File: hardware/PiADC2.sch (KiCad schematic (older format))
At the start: 1 part

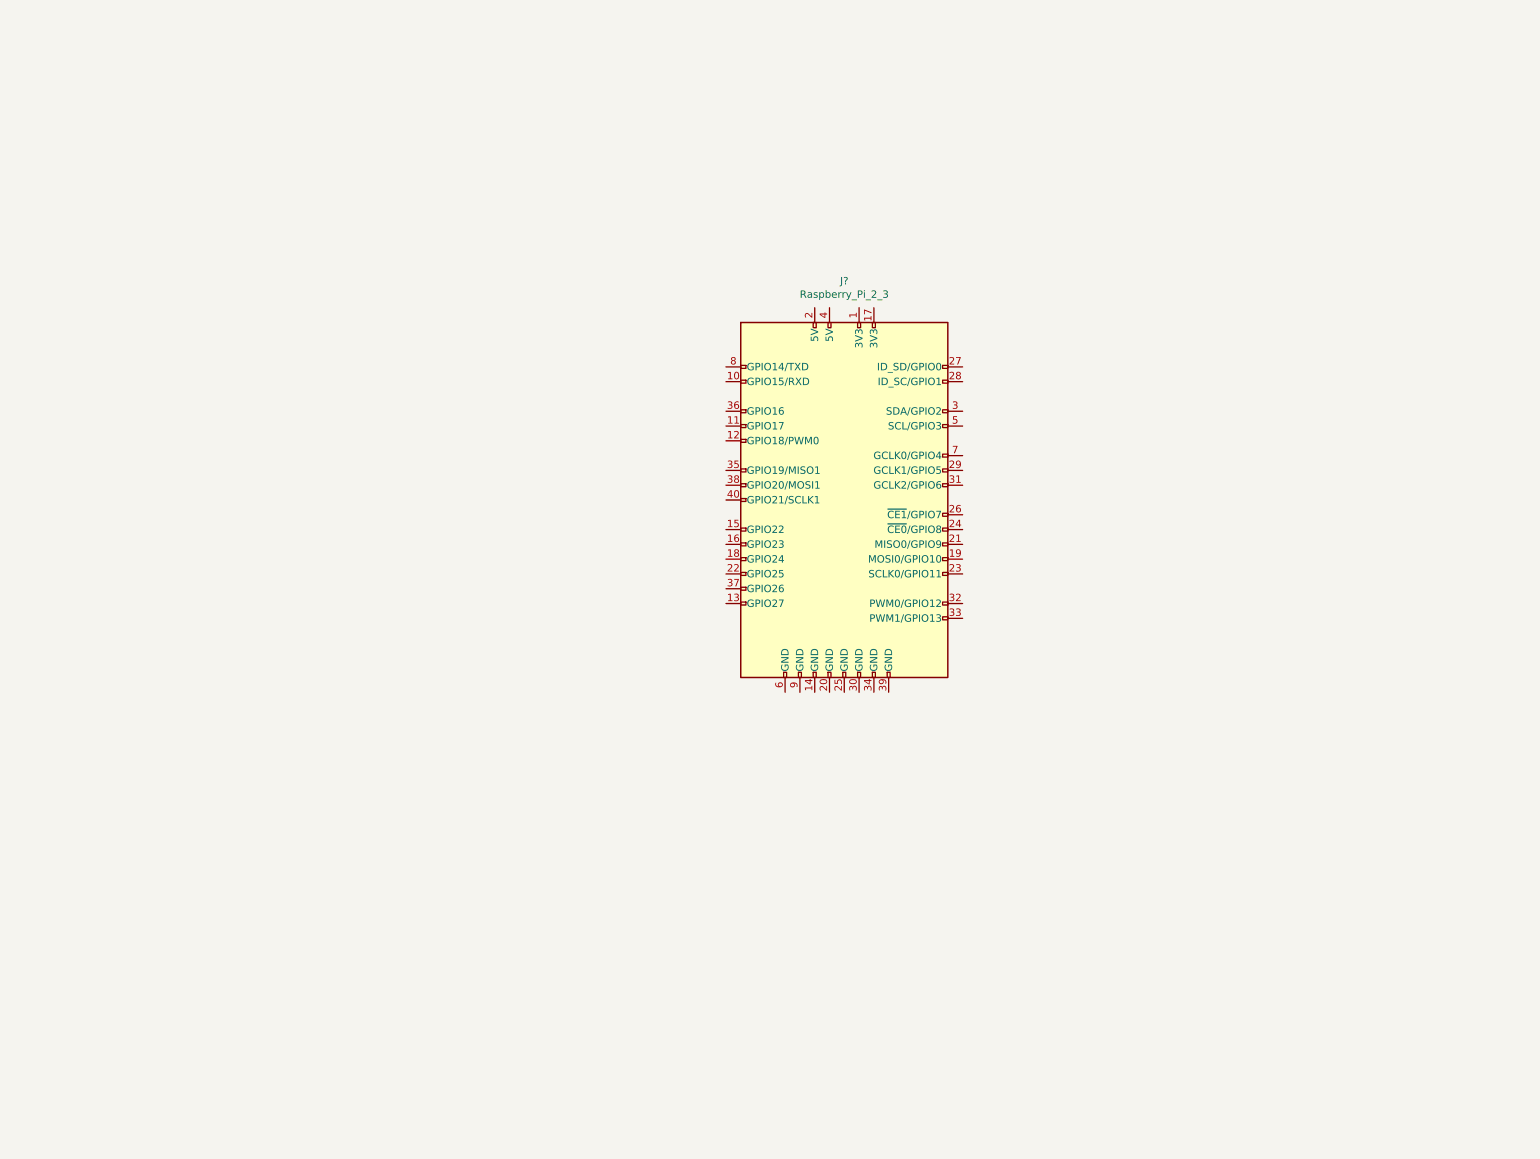
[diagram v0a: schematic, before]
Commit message: Completed version 1
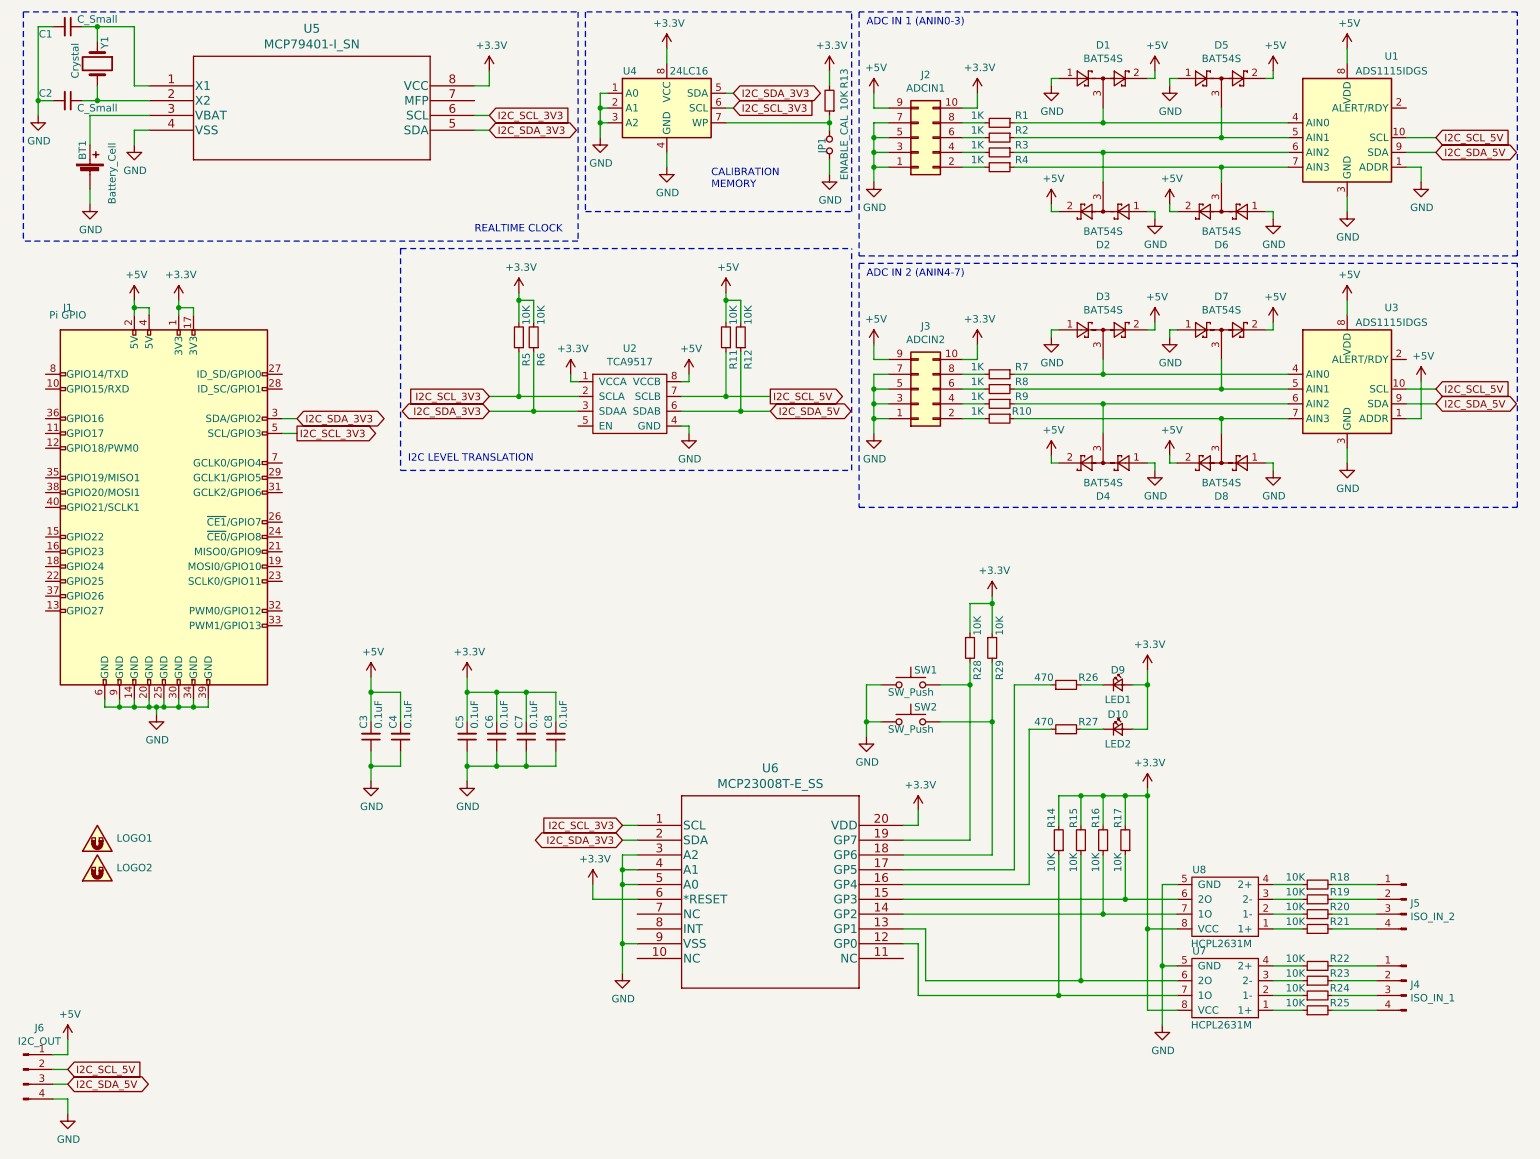
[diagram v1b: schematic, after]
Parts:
- added BT1: Battery_Cell, BH401:BH401, symbol Device:Battery_Cell
- added C1, C2: C_Small, Capacitor_SMD:C_0603_1608Metric, symbol Device:C_Small
- added C3, C4, C5, C6, C7, C8: 0.1uF, Capacitor_SMD:C_0603_1608Metric, symbol Device:C_Small
- added D1, D2, D3, D4, D5, D6, D7, D8: BAT54S, Package_TO_SOT_SMD:SOT-23, symbol Diode:BAT54S
- added D10: LED2, LED_SMD:LED_0603_1608Metric, symbol Device:LED_Small
- added D9: LED1, LED_SMD:LED_0603_1608Metric, symbol Device:LED_Small
- added J2: ADCIN1, Connector_JST:JST_PUD_B10B-PUDSS_2x05_P2.00mm_Vertical, symbol Connector_Generic:Conn_02x05_Odd_Even
- added J3: ADCIN2, Connector_JST:JST_PUD_B10B-PUDSS_2x05_P2.00mm_Vertical, symbol Connector_Generic:Conn_02x05_Odd_Even
- added J4: ISO_IN_1, JST-XA:B04B-XASK-1(LF)(SN), symbol Connector:Conn_01x04_Male
- added J5: ISO_IN_2, JST-XA:B04B-XASK-1(LF)(SN), symbol Connector:Conn_01x04_Male
- added J6: I2C_OUT, Connector_PinHeader_2.54mm:PinHeader_1x04_P2.54mm_Vertical, symbol Connector:Conn_01x04_Male
- added JP1: ENABLE_CAL, Connector_PinHeader_1.27mm:PinHeader_1x02_P1.27mm_Vertical, symbol Device:Jumper_NO_Small
- added LOGO1: SYM_Magnet_Small, CapConiX_Logos:CapConiX_Logo_10_7, symbol Graphic:SYM_Magnet_Small
- added LOGO2: SYM_Magnet_Small, Symbol:OSHW-Logo_5.7x6mm_SilkScreen, symbol Graphic:SYM_Magnet_Small
- added R1, R10, R2, R3, R4, R7, R8, R9: 1K, Resistor_SMD:R_0603_1608Metric, symbol Device:R_Small
- added R11, R12, R13, R14, R15, R16, R17, R18, R19, R20, R21, R22, R23, R24, R25, R28, R29, R5, R6: 10K, Resistor_SMD:R_0603_1608Metric, symbol Device:R_Small
- added R26, R27: 470, Resistor_SMD:R_0603_1608Metric, symbol Device:R_Small
- added SW1, SW2: SW_Push, Button_Switch_SMD:SW_SPST_TL3305A, symbol Switch:SW_Push
- added U1, U3: ADS1115IDGS, Package_SO:TSSOP-10_3x3mm_P0.5mm, symbol Analog_ADC:ADS1115IDGS
- added U2: TCA9517, Package_SO:MSOP-8_3x3mm_P0.65mm, symbol tca9517:TCA9517
- added U4: 24LC16, Package_SO:SO-8_3.9x4.9mm_P1.27mm, symbol Memory_EEPROM:24LC16
- added U5: MCP79401-I_SN, Package_SO:SO-8_3.9x4.9mm_P1.27mm, symbol MCP79401:MCP79401-I_SN
- added U6: MCP23008T-E_SS, Package_SO:SSOP-20_5.3x7.2mm_P0.65mm, symbol MCP23008:MCP23008T-E_SS
- added U7, U8: HCPL2631M, Package_DIP:DIP-8_W7.62mm_LongPads, symbol HCPL2631M:HCPL2631M
- added Y1: Crystal, Crystal:Crystal_DS26_D2.0mm_L6.0mm_Horizontal_1EP_style2, symbol Device:Crystal
- J1: renamed from J?; value Raspberry_Pi_2_3 -> Pi GPIO; footprint (none) -> raspberry_pi:pi_b_hat
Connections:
- net +3V3: now reaches J1.1 (3V3)
- net +3V3: now also J1.17 (3V3), C5.2, C6.2, C7.2, C8.2, D10.2 (A), D9.2 (A), J2.10 (Pin_10), J3.10 (Pin_10), R13.2, R14.2, R15.2, R16.2, R17.2, R28.1, R29.1, R5.2, R6.2, U2.1 (VCCA), U4.8 (VCC), U5.8 (VCC), U6.20 (VDD), U6.6 (*RESET), U7.8 (VCC), U8.8 (VCC)
- net GND: now reaches J1.14 (GND)
- net GND: now also J1.20 (GND), J1.25 (GND), J1.30 (GND), J1.34 (GND), J1.39 (GND), J1.6 (GND), J1.9 (GND), BT1.2 (-), C1.2, C2.2, C3.1, C4.1, C5.1, C6.1, C7.1, C8.1, D1.1, D2.1, D3.1, D4.1, D5.1, D6.1, D7.1, D8.1, J2.1 (Pin_1), J2.3 (Pin_3), J2.5 (Pin_5), J2.7 (Pin_7), J3.1 (Pin_1), J3.3 (Pin_3), J3.5 (Pin_5), J3.7 (Pin_7), J6.4 (Pin_4), JP1.2, SW1.1, SW2.1, U1.1 (ADDR), U1.3 (GND), U2.4 (GND), U3.3 (GND), U4.1 (A0), U4.2 (A1), U4.3 (A2), U4.4 (GND), U5.4 (VSS), U6.3 (A2), U6.4 (A1), U6.5 (A0), U6.9 (VSS), U7.5 (GND), U8.5 (GND)
- net +5V: now reaches J1.2 (5V)
- net +5V: now also J1.4 (5V), C3.2, C4.2, D1.2, D2.2, D3.2, D4.2, D5.2, D6.2, D7.2, D8.2, J2.9 (Pin_9), J3.9 (Pin_9), J6.1 (Pin_1), R11.2, R12.2, U1.8 (VDD), U2.8 (VCCB), U3.1 (ADDR), U3.8 (VDD)
- net I2C_SDA_3V3: now reaches J1.3 (SDA/GPIO2)
- net I2C_SDA_3V3: now also R6.1, U2.3 (SDAA), U4.5 (SDA), U5.5 (SDA), U6.2 (SDA)
- net I2C_SCL_3V3: now reaches J1.5 (SCL/GPIO3)
- net I2C_SCL_3V3: now also R5.1, U2.2 (SCLA), U4.6 (SCL), U5.6 (SCL), U6.1 (SCL)
- new net: J2.2 (Pin_2), R4.2
- new net: J2.4 (Pin_4), R3.2
- new net: J2.6 (Pin_6), R2.2
- new net: J2.8 (Pin_8), R1.2
- new net: D1.3, R1.1, U1.4 (AIN0)
- new net: D5.3, R2.1, U1.5 (AIN1)
- new net: D2.3, R3.1, U1.6 (AIN2)
- new net: D6.3, R4.1, U1.7 (AIN3)
- new net: JP1.1, R13.1, U4.7 (WP)
- new net: C1.1, U5.1 (X1), Y1.1
- new net: C2.1, U5.2 (X2), Y1.2
- new net: BT1.1 (+), U5.3 (VBAT)
- new net: R14.1, U6.12 (GP0), U7.7 (1O)
- new net: R15.1, U6.13 (GP1), U7.6 (2O)
- new net: R16.1, U6.14 (GP2), U8.7 (1O)
- new net: R17.1, U6.15 (GP3), U8.6 (2O)
- new net: R27.1, U6.16 (GP4)
- new net: R26.1, U6.17 (GP5)
- new net: R29.2, SW2.2, U6.18 (GP6)
- new net: R28.2, SW1.2, U6.19 (GP7)
- new net: J3.2 (Pin_2), R10.2
- new net: J3.4 (Pin_4), R9.2
- new net: J3.6 (Pin_6), R8.2
- new net: J3.8 (Pin_8), R7.2
- new net: D3.3, R7.1, U3.4 (AIN0)
- new net: D7.3, R8.1, U3.5 (AIN1)
- new net: D4.3, R9.1, U3.6 (AIN2)
- new net: D8.3, R10.1, U3.7 (AIN3)
- new net: R25.1, U7.1 (1+)
- new net: R24.1, U7.2 (1-)
- new net: R23.1, U7.3 (2-)
- new net: R22.1, U7.4 (2+)
- new net: R21.1, U8.1 (1+)
- new net: R20.1, U8.2 (1-)
- new net: R19.1, U8.3 (2-)
- new net: R18.1, U8.4 (2+)
- new net: J4.1 (Pin_1), R22.2
- new net: J4.2 (Pin_2), R23.2
- new net: J4.3 (Pin_3), R24.2
- new net: J4.4 (Pin_4), R25.2
- new net: J5.4 (Pin_4), R21.2
- new net: J5.3 (Pin_3), R20.2
- new net: J5.2 (Pin_2), R19.2
- new net: J5.1 (Pin_1), R18.2
- new net: D9.1 (K), R26.2
- new net: D10.1 (K), R27.2
- new net I2C_SCL_5V: J6.2 (Pin_2), R11.1, U1.10 (SCL), U2.7 (SCLB), U3.10 (SCL)
- new net I2C_SDA_5V: J6.3 (Pin_3), R12.1, U1.9 (SDA), U2.6 (SDAB), U3.9 (SDA)
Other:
- note added: "ADC IN 1 (ANIN0-3)"
- note added: "ADC IN 2 (ANIN4-7)"
- note added: "CALIBRATION\nMEMORY"
- note added: "I2C LEVEL TRANSLATION"
- note added: "REALTIME CLOCK"
- moved on the sheet: J1
